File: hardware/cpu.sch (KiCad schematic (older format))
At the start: 41 parts

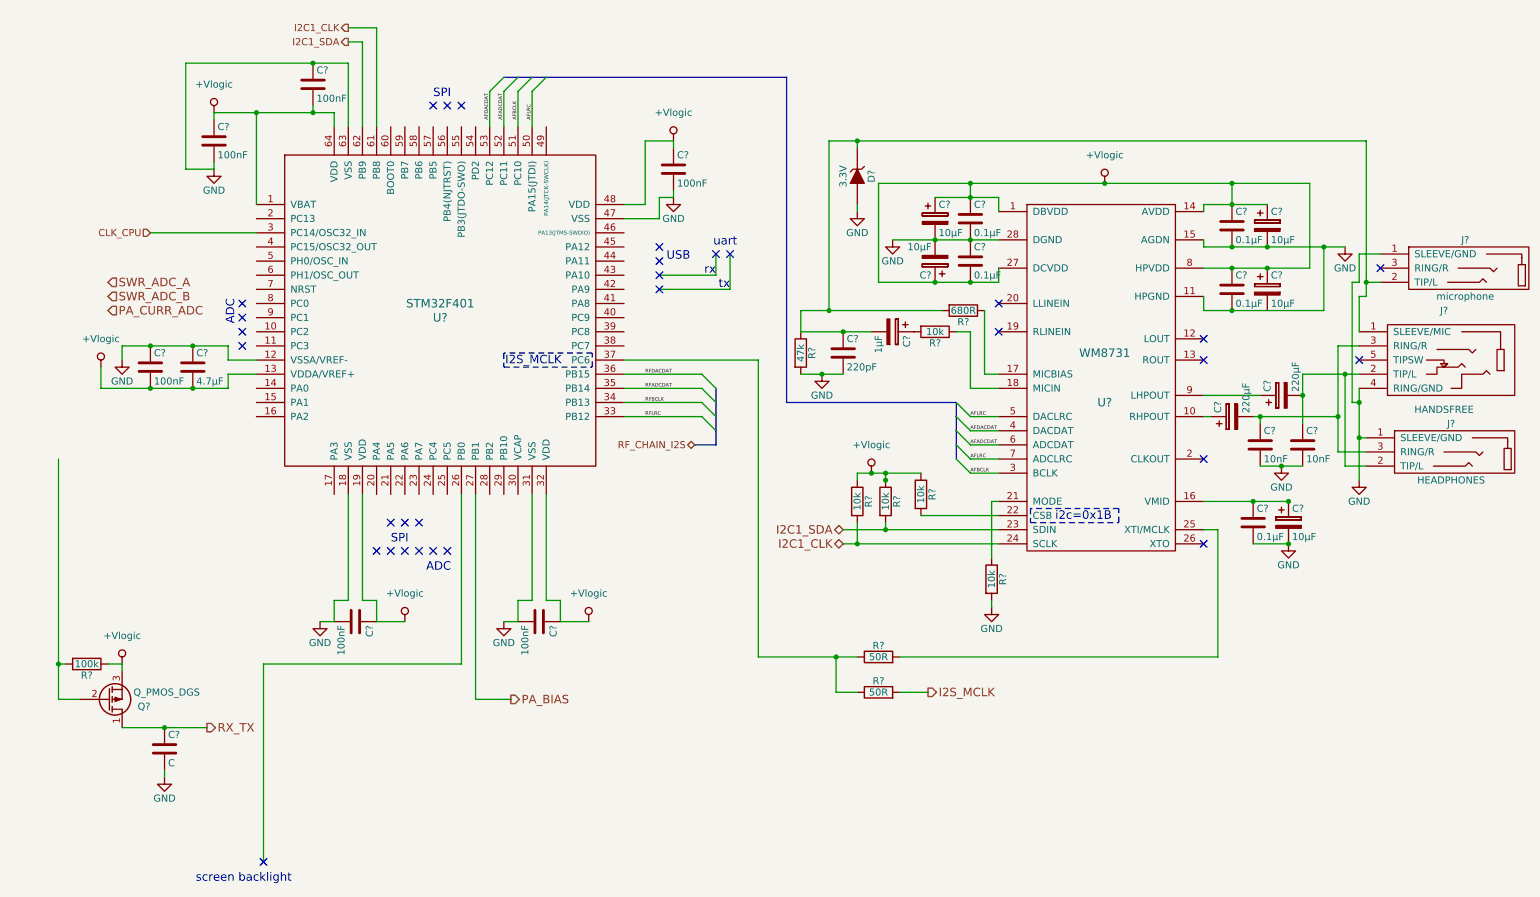
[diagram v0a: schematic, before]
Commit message: Made some minor adjustments and replotted schematic .pdf
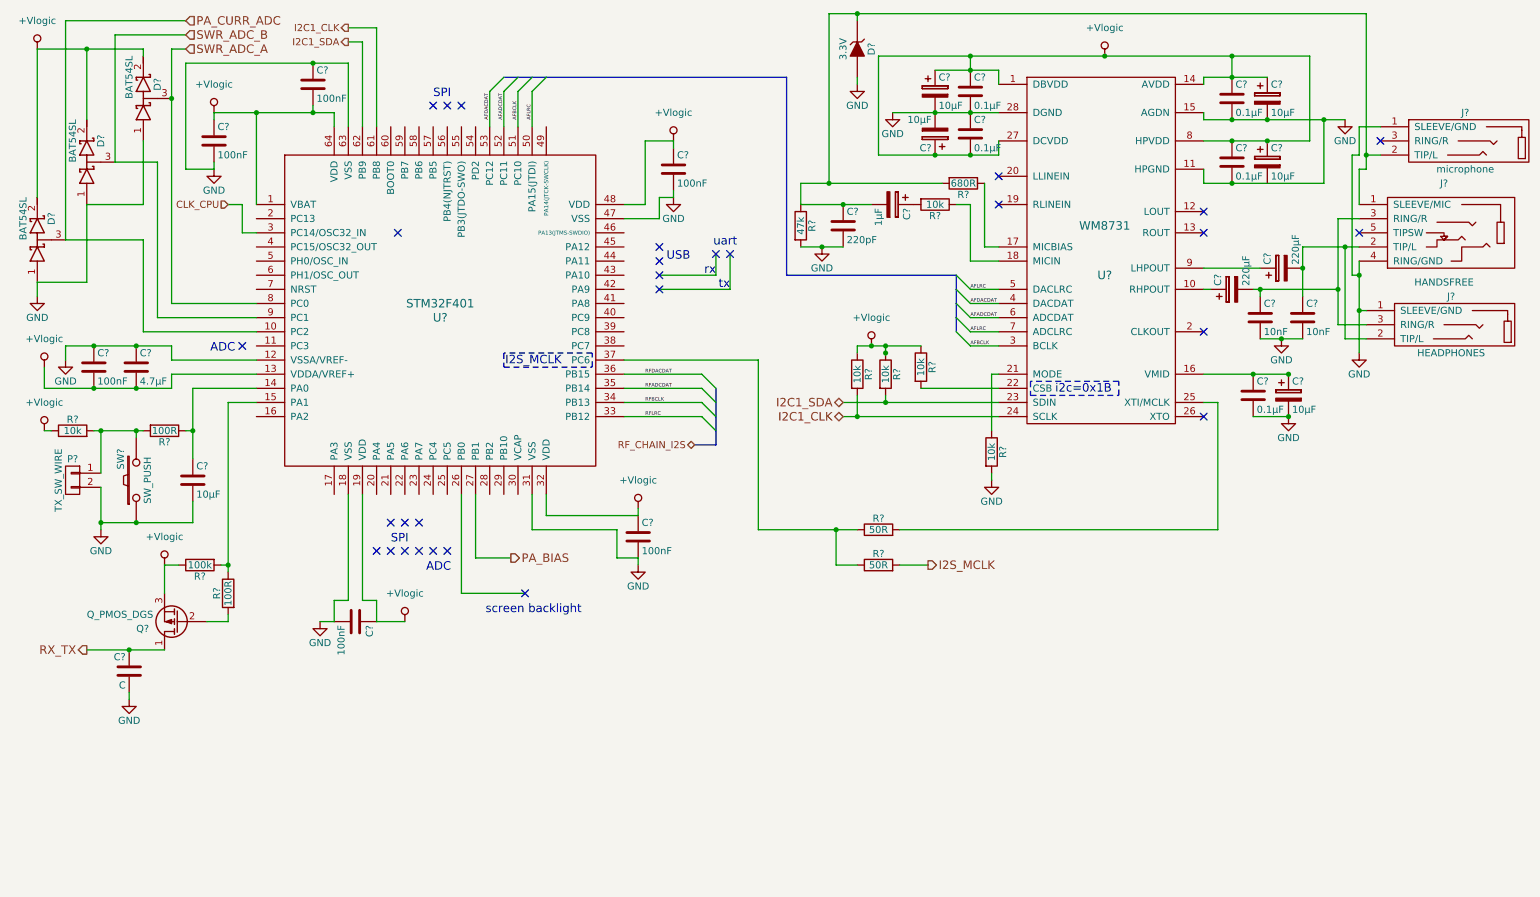
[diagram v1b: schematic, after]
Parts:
- added C?: 10µF, symbol C
- added D? (x3): BAT54SL, symbol D_Schottky_x2_Serial_AKC
- added P?: TX_SW_WIRE, symbol CONN_01X02
- added R?: 10k, symbol R
- added R? (x2): 100R, symbol R
- added SW?: SW_PUSH, symbol SW_PUSH
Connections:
- net +Vlogic: now also D?.2 (K), D?.2 (K), D?.2 (K), R?.1
- net GND: now also C?.2, D?.1 (A), D?.1 (A), D?.1 (A), P?.2 (P2), SW?.1
- net PA_CURR_ADC: now also U?.10 (PC2), D?.3 (common)
- net SWR_ADC_A: now also U?.8 (PC0), D?.3 (common)
- net SWR_ADC_B: now also U?.9 (PC1), D?.3 (common)
- net at U?.14 (PA0): now also C?.1, R?.1
- net at U?.15 (PA1): now also R?.2, R?.1
- net at Q?.2 (G): now also R?.2; no longer R?.2
- new net: P?.1 (P1), R?.2, R?.2, SW?.2
- no-connect marks 31 -> 29
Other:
- moved on the sheet: C?, D?, J?, Q?, R?, U?

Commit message: fixed some bugs
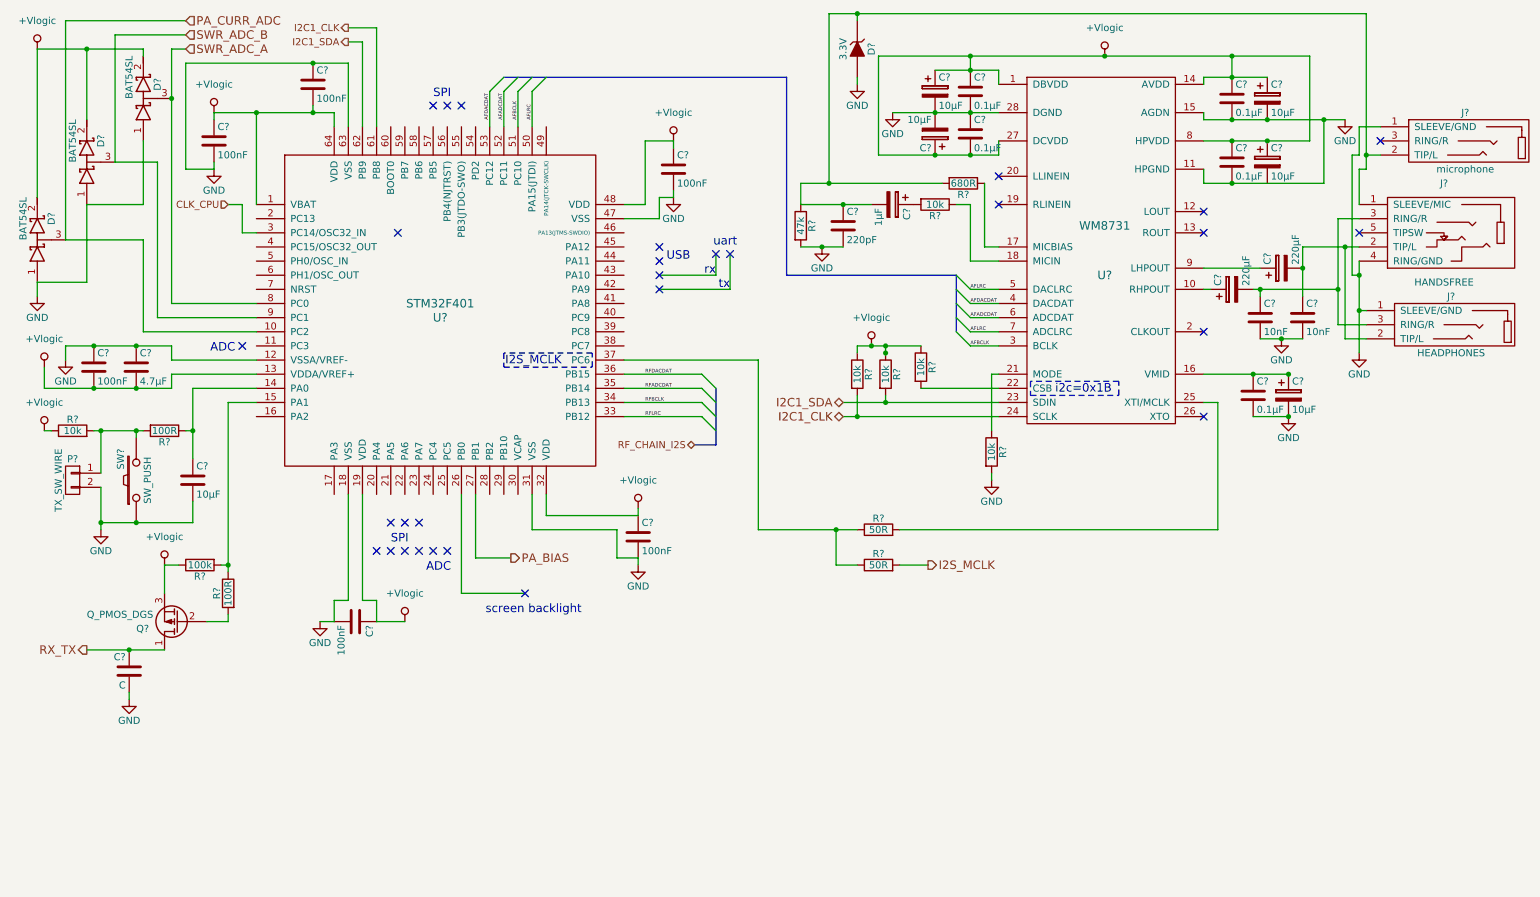
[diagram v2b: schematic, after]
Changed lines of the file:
@@
 NoConn ~ 10000 2100
 Wire Wire Line
-	1900 1250 2200 1250
-Wire Wire Line
-	2200 1250 2600 1250
-Wire Wire Line
-	2600 1250 2750 1250
+	1900 1250 2750 1250
 Wire Wire Line
 	2750 1250 2750 1350
@@
 	2850 900  2850 1350
 Wire Wire Line
-	1700 900  2600 900
-Wire Wire Line
-	2600 900  2850 900
+	1700 900  2850 900
 Wire Wire Line
 	1700 900  1700 1650
@@
 	2200 3100 1600 3100
 Wire Wire Line
-	1600 3100 1600 3200
-Wire Wire Line
-	1600 3200 1350 3200
-Wire Wire Line
-	1350 3200 1050 3200
-Wire Wire Line
-	1050 3200 700  3200
+	1600 3200 1600 3100
+Wire Wire Line
+	700  3200 1600 3200
 Wire Wire Line
 	700  3200 700  3050
@@
 	850  3000 850  2900
 Wire Wire Line
-	850  2900 1050 2900
-Wire Wire Line
-	1050 2900 1350 2900
-Wire Wire Line
-	1350 2900 1600 2900
+	850  2900 1600 2900
 Wire Wire Line
 	1600 2900 1600 3000
@@
 Connection ~ 1350 3200
 Wire Wire Line
-	6700 1250 7000 1250
-Wire Wire Line
-	7000 1250 7250 1250
-Wire Wire Line
-	7250 1250 7450 1250
+	6700 1250 7450 1250
 Wire Wire Line
 	7450 950  7450 1050
 Wire Wire Line
-	7000 950  7250 950
-Wire Wire Line
-	7250 950  7450 950
+	7000 950  7450 950
 Connection ~ 7250 950
 Wire Wire Line
 	7250 950  7250 850
 Wire Wire Line
-	6600 850  7250 850
-Wire Wire Line
-	7250 850  8200 850
-Wire Wire Line
-	8200 850  9100 850
-Wire Wire Line
-	9100 850  9650 850
+	6600 850  9650 850
 Connection ~ 7000 1250
 Connection ~ 7250 1250
@@
 Connection ~ 8200 850
 Wire Wire Line
-	8900 1000 9100 1000
-Wire Wire Line
-	9100 1000 9350 1000
+	8900 1000 9350 1000
 Wire Wire Line
 	8900 1000 8900 1050
 Connection ~ 9100 1000
 Wire Wire Line
-	8900 1300 9100 1300
-Wire Wire Line
-	9100 1300 9350 1300
-Wire Wire Line
-	9350 1300 9750 1300
-Wire Wire Line
-	9750 1300 9900 1300
+	8900 1300 9900 1300
 Wire Wire Line
 	8900 1300 8900 1250
@@
 Connection ~ 9350 1300
 Wire Wire Line
-	9650 850  9650 1450
-Wire Wire Line
-	9650 1450 9350 1450
-Wire Wire Line
-	9350 1450 9100 1450
-Wire Wire Line
-	9100 1450 8900 1450
+	9650 1450 9650 850
+Wire Wire Line
+	8900 1450 9650 1450
 Connection ~ 9100 850
 Connection ~ 9350 1450
@@
 	8900 1650 8900 1750
 Wire Wire Line
-	8900 1750 9100 1750
-Wire Wire Line
-	9100 1750 9750 1750
+	8900 1750 9750 1750
 Wire Wire Line
 	9750 1750 9750 1300
@@
 Connection ~ 9100 1750
 Wire Wire Line
-	6600 1550 7000 1550
-Wire Wire Line
-	7000 1550 7250 1550
-Wire Wire Line
-	7250 1550 7450 1550
+	6600 1550 7450 1550
 Wire Wire Line
 	7450 1550 7450 1450
@@
 Connection ~ 7000 1550
 Wire Wire Line
-	6350 3300 6650 3300
-Wire Wire Line
-	6650 3300 7450 3300
+	6350 3300 7450 3300
 Wire Wire Line
 	6650 3300 6650 3250
 Wire Wire Line
-	6350 3400 6450 3400
-Wire Wire Line
-	6450 3400 7450 3400
+	6350 3400 7450 3400
 Wire Wire Line
 	6450 3400 6450 3250
@@
 Connection ~ 6650 2950
 Wire Wire Line
-	6450 2900 6550 2900
-Wire Wire Line
-	6550 2900 6650 2900
-Wire Wire Line
-	6650 2900 6900 2900
+	6450 2900 6900 2900
 Wire Wire Line
 	6450 2900 6450 2950
@@
 	7400 3100 7400 3500
 Wire Wire Line
-	5750 4200 6300 4200
-Wire Wire Line
-	6300 4200 6450 4200
+	5750 4200 6450 4200
 Wire Wire Line
 	5750 4200 5750 3000
@@
 	7250 2900 7450 2900
 Wire Bus Line
-	7150 2400 7150 2500
-Wire Bus Line
-	7150 2500 7150 2600
-Wire Bus Line
-	7150 2600 7150 2700
-Wire Bus Line
-	7150 2700 7150 2800
+	7150 2400 7150 2800
 Wire Bus Line
 	5950 2400 7150 2400
@@
 	5950 1000 5950 2400
 Wire Bus Line
-	3950 1000 4050 1000
-Wire Bus Line
-	4050 1000 4150 1000
-Wire Bus Line
-	4150 1000 4250 1000
-Wire Bus Line
-	4250 1000 5950 1000
+	3950 1000 5950 1000
 Wire Wire Line
 	2850 750  2950 750
@@
 	3050 650  3050 1350
 Wire Wire Line
-	9300 2850 9450 2850
-Wire Wire Line
-	9450 2850 9600 2850
+	9300 2850 9600 2850
 Connection ~ 9450 2850
 Wire Wire Line
 	9250 3400 9500 3400
 Wire Wire Line
-	8900 3100 9250 3100
-Wire Wire Line
-	9250 3100 9500 3100
-Wire Wire Line
-	9600 2200 9600 2350
-Wire Wire Line
-	9600 2350 9600 2550
-Wire Wire Line
-	9600 2200 9900 2200
-Wire Wire Line
-	9900 2200 10000 2200
+	8900 3100 9500 3100
+Wire Wire Line
+	9600 2200 9600 2550
+Wire Wire Line
+	9600 2200 10000 2200
 Wire Wire Line
 	9850 2000 10000 2000
 Wire Wire Line
-	9250 2500 9300 2500
-Wire Wire Line
-	9300 2500 9850 2500
-Wire Wire Line
-	9850 2000 9850 2500
-Wire Wire Line
-	9850 2500 9850 2750
+	9250 2500 9850 2500
+Wire Wire Line
+	9850 2000 9850 2750
 Wire Wire Line
 	9900 2200 9900 2850
@@
 	10000 2650 10050 2650
 Wire Wire Line
-	10000 2300 10000 2400
-Wire Wire Line
-	10000 2400 10000 2650
-Wire Wire Line
-	10000 2650 10000 2950
+	10000 2300 10000 2950
 Connection ~ 10000 2650
 Wire Wire Line
@@
 Connection ~ 10050 1550
 Wire Wire Line
-	10050 550  10050 1550
-Wire Wire Line
-	10050 1550 10050 1650
-Wire Wire Line
-	6250 550  6450 550
-Wire Wire Line
-	6450 550  10050 550
+	10050 550  10050 1650
+Wire Wire Line
+	6250 550  10050 550
 Connection ~ 9850 2500
 Wire Wire Line
@@
 	6850 1900 6850 1900
 Wire Wire Line
-	6050 1750 6250 1750
-Wire Wire Line
-	6250 1750 7050 1750
+	6050 1750 7050 1750
 Wire Wire Line
 	6050 1750 6050 1900
 Wire Wire Line
-	6050 1900 6350 1900
-Wire Wire Line
-	6350 1900 6550 1900
+	6050 1900 6550 1900
 Connection ~ 6350 1900
 $Comp
@@
 $EndComp
 Wire Wire Line
-	6050 2200 6200 2200
-Wire Wire Line
-	6200 2200 6350 2200
+	6050 2200 6350 2200
 Connection ~ 6200 2200
 Wire Wire Line
@@
 RF_CHAIN_I2S
 Wire Bus Line
-	5450 3200 5450 3300
-Wire Bus Line
-	5450 3300 5450 3400
-Wire Bus Line
-	5450 3400 5450 3500
-Wire Bus Line
-	5450 3500 5450 3600
+	5450 3200 5450 3600
 Wire Bus Line
 	5450 3600 5300 3600
@@
 	1300 5400 1300 5350
 Wire Wire Line
-	1000 5050 1300 5050
-Wire Wire Line
-	1300 5050 1550 5050
+	1000 5050 1550 5050
 Connection ~ 1300 5050
 $Comp
@@
 $EndComp
 Wire Wire Line
-	1050 3500 1100 3500
-Wire Wire Line
-	1100 3500 1350 3500
-Wire Wire Line
-	1350 3500 1400 3500
+	1050 3500 1400 3500
 Wire Wire Line
 	1350 3500 1350 3550
@@
 $EndComp
 Wire Wire Line
-	1750 3200 1750 3500
-Wire Wire Line
-	1750 3500 1750 3700
+	1750 3200 1750 3700
 Connection ~ 1750 3500
 Wire Wire Line
 	1750 4150 1750 4000
 Wire Wire Line
-	1100 4150 1350 4150
-Wire Wire Line
-	1350 4150 1750 4150
+	1100 4150 1750 4150
 Wire Wire Line
 	1100 3500 1100 3800
 Wire Wire Line
-	1100 3900 1100 4150
-Wire Wire Line
-	1100 4150 1100 4200
+	1100 3900 1100 4200
 Connection ~ 1350 4150
 Wire Wire Line
@@
 Connection ~ 1100 3500
 Wire Wire Line
-	2000 3300 2000 4450
-Wire Wire Line
-	2000 4450 2000 4500
+	2000 3300 2000 4500
 Wire Wire Line
 	4250 4100 4250 3950
@@
 	1600 2600 2200 2600
 Wire Wire Line
-	1600 800  1600 1150
-Wire Wire Line
-	1600 1150 1600 2600
+	1600 800  1600 2600
 Wire Wire Line
 	1400 2150 850  2150
@@
 $EndComp
 Wire Wire Line
-	650  800  1000 800
-Wire Wire Line
-	1000 800  1400 800
+	650  800  1400 800
 Wire Wire Line
 	1400 800  1400 850
